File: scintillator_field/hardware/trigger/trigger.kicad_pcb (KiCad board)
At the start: 2 copper layers, 110 parts, among them J1 Conn_02x03_Top_Bottom, J2 Conn_02x03_Top_Bottom, J3 A1, J4 A2, J5 A3, J6 Conn_Coaxial_Small, J7 Conn_02x03_Top_Bottom, J8 Conn_02x03_Top_Bottom, J9 Conn_Coaxial_Small, U1 LT3461A, U10 OPA855xDSG, U11 TLV3501AIDBV, U2 TPS7A4701, U3 TPS7A4701, U4 OPA855xDSG, U5 TLV3501AIDBV, U6 OPA855xDSG, U7 TLV3501AIDBV, U8 OPA855xDSG, U9 TLV3501AIDBV

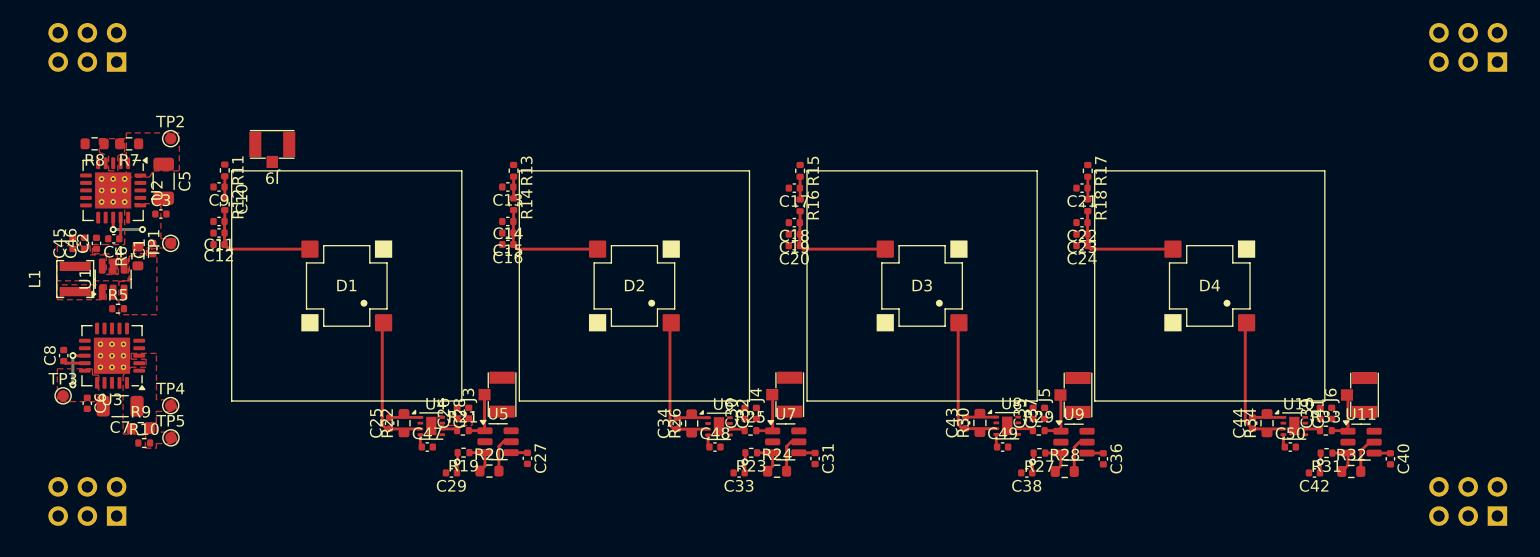
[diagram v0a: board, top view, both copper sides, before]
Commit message: finalize pcb
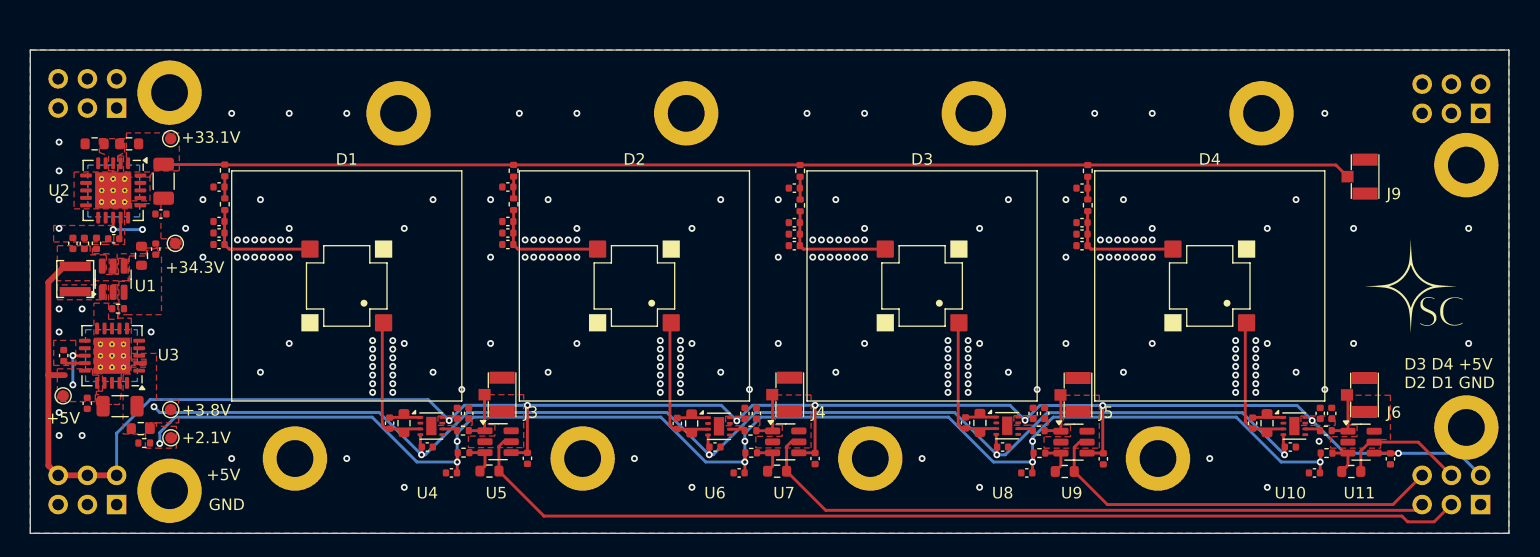
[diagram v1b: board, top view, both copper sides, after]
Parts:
- added ?: , , F.Cu at (84.6, 83.2)
- added ?: , , F.Cu at (129.5, 85.0)
- added ?: , , F.Cu at (84.6, 117.8)
- added ?: , , F.Cu at (104.5, 85.0)
- added ?: , , F.Cu at (179.5, 85.0)
- added ?: , , F.Cu at (154.5, 85.0)
- added ?: , , F.Cu at (197.3, 89.5)
- added ?: , , F.Cu at (145.5, 115.0)
- added ?: , , F.Cu at (170.5, 115.0)
- added ?: , , F.Cu at (197.3, 112.3)
- added ?: , , F.Cu at (120.5, 115.0)
- added G***: LOGO, logos:sc, F.Cu at (192.5, 100.0)
- added G***: LOGO, logos:hep_14mm, B.Cu at (81.5, 95.5)
- added REF**: MountingHole_3.2mm_M3_DIN965_Pad, MountingHole:MountingHole_3.2mm_M3_DIN965_Pad, F.Cu at (95.5, 115.0)
- moved J9 95.0 mm to (188.5, 90.5), turned to 90 degrees
- moved J7 4.69 mm to (198.5, 85.0)
- moved J8 4.00 mm to (80.0, 84.5)
- moved J1 1.77 mm to (198.5, 119.0)
- moved J2 1.00 mm to (80.0, 119.0)
- moved +34.3V 0.40 mm to (85.1, 96.3)
- moved +3.8V 0.35 mm to (84.7, 110.8)
- moved R6 0.31 mm to (82.2, 97.4)
- moved C1 0.25 mm to (83.4, 96.8)
- renumbered TP5 to +2.1V, TP4 to +3.8V, TP2 to +33.1V, TP1 to +34.3V, TP3 to +5V
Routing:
- net +5V: track 9.27 -> 178.4 mm, vias 2 -> 10
- net +2.1V: track 7.08 -> 124.9 mm, vias 4 -> 8
- net +3.8V: track 4.48 -> 116.4 mm, vias 0 -> 5
- net +33.1V: track 0.00 -> 103.3 mm
- net /amplifiers/DOUT1: track 3.38 -> 88.6 mm
- net /amplifiers/DOUT2: track 3.38 -> 60.9 mm
- net /amplifiers/DOUT3: track 3.40 -> 35.9 mm
- net /amplifiers/DOUT4: track 3.26 -> 11.2 mm
- net GND: track 0.00 -> 0.49 mm, vias 0 -> 195
- added copper zone on B.Cu, net GND
- added copper zone on F.Cu, net GND
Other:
- board outline added: 128.5 x 42 mm
- board text added: "+5V"
- board text added: "ALEX X ENRICHED P&E 2025/03/16"
- board text added: "D1"
- board text added: "D2"
- board text added: "D3"
- board text added: "D3 D4 +5V D2 D1 GND"
- board text added: "D4"
- board text added: "GND"
